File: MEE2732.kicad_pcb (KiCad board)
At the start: 2 copper layers, 32.9 x 16.6 mm, 6 parts, among them J1 Molex 78805 socket with 27C32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, SW1 SW_SPDT, U1 28C64 / FM16W08

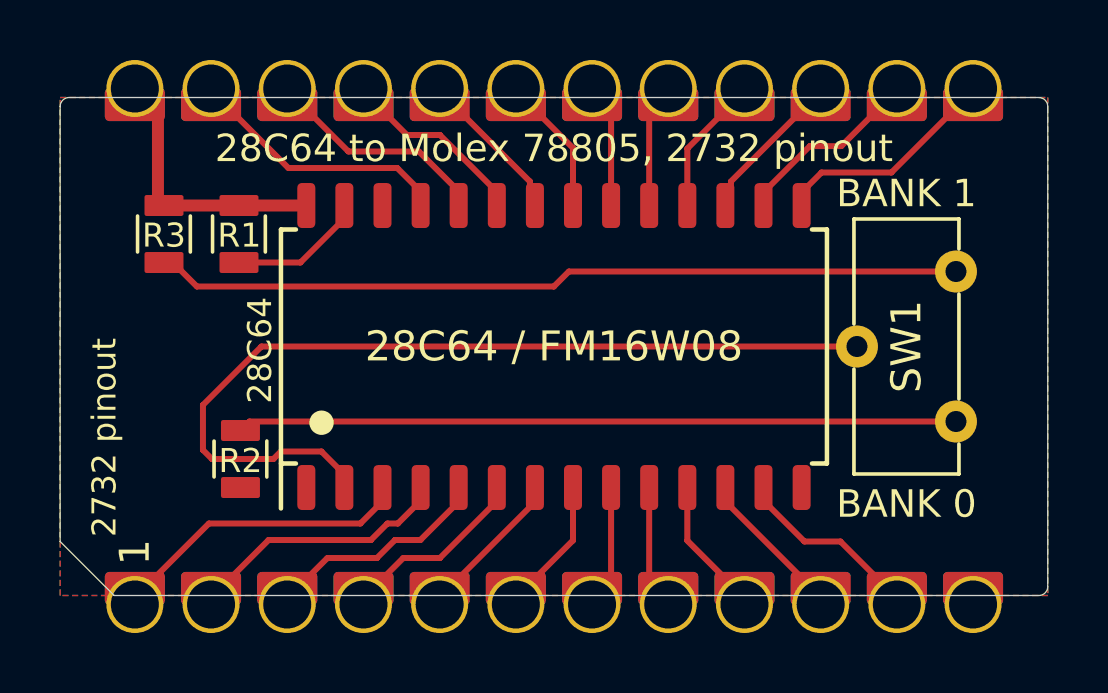
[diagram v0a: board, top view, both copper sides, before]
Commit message: MEE2732 minor tidy up
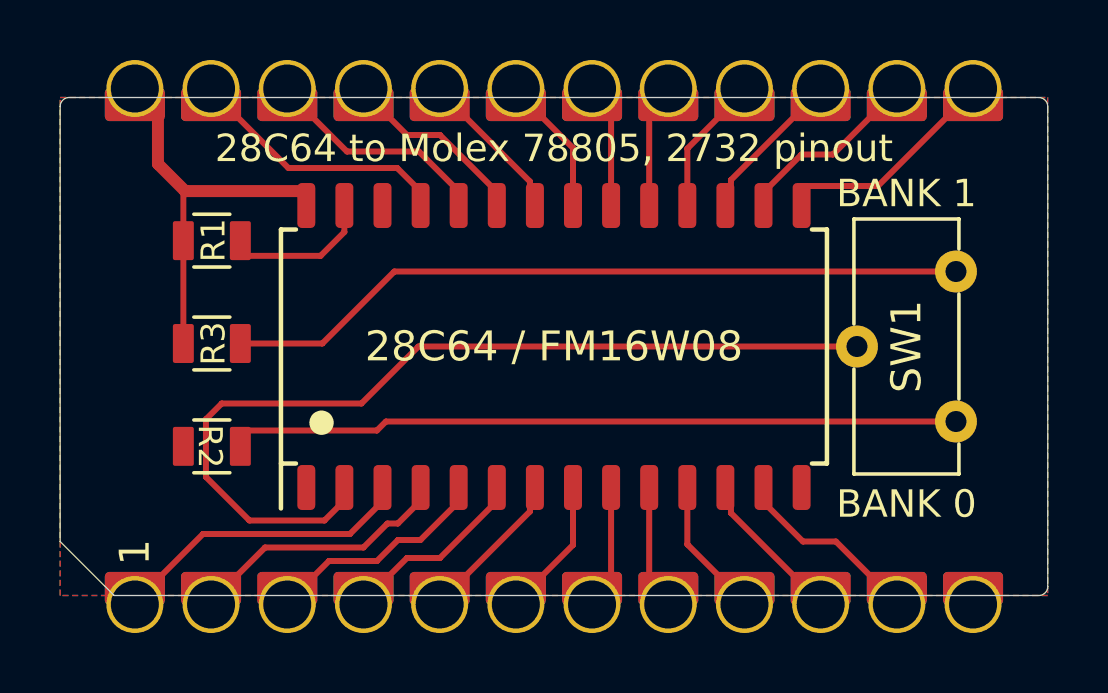
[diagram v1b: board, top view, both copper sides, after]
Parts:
- moved R3 3.98 mm to (135.9, 99.2), turned to 180 degrees
- moved R2 1.04 mm to (135.9, 102.6), turned to 180 degrees
- moved R1 0.93 mm to (135.9, 95.8), turned to 180 degrees
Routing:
- net VCC: track 9.05 -> 13.7 mm
- net Net-(R3-Pad1): track 26.9 -> 24.8 mm
- net /A12: track 29.8 -> 30.6 mm
- net /~{WE}: track 4.56 -> 5.19 mm
- net Net-(R2-Pad1): track 24.0 -> 24.5 mm
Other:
- board text removed: "2732 pinout"
- board text removed: "28C64"
